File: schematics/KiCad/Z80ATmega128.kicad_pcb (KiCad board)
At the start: 2 copper layers, 97 parts, among them J1 AVR-ISP-6, J2 DC 5V, J3 DC 5V, J4 Z80[1..20], J5 Z80[21..40], J6 Micro_SD_Card_Det_Hirose_DM3AT, SW1 POWER, SW2 RESET, SW3 RESET, U1 74HC125, U10 AE-CH340E-TYPEC, U11 74HC08, U12 74HC32, U13 74HC74, U14 DS1232, U15 74HC132, U16 74HC4050, U17 LP2950-3.3, U2 74AC573, U3 74HCT574, U4 74HC04, U5 AE-CH340E-TYPEC, U6 74HC125, U7 74HC244, U8 74HCT245, U9 74HC32, Y1 16MHz, Y2 8MHz

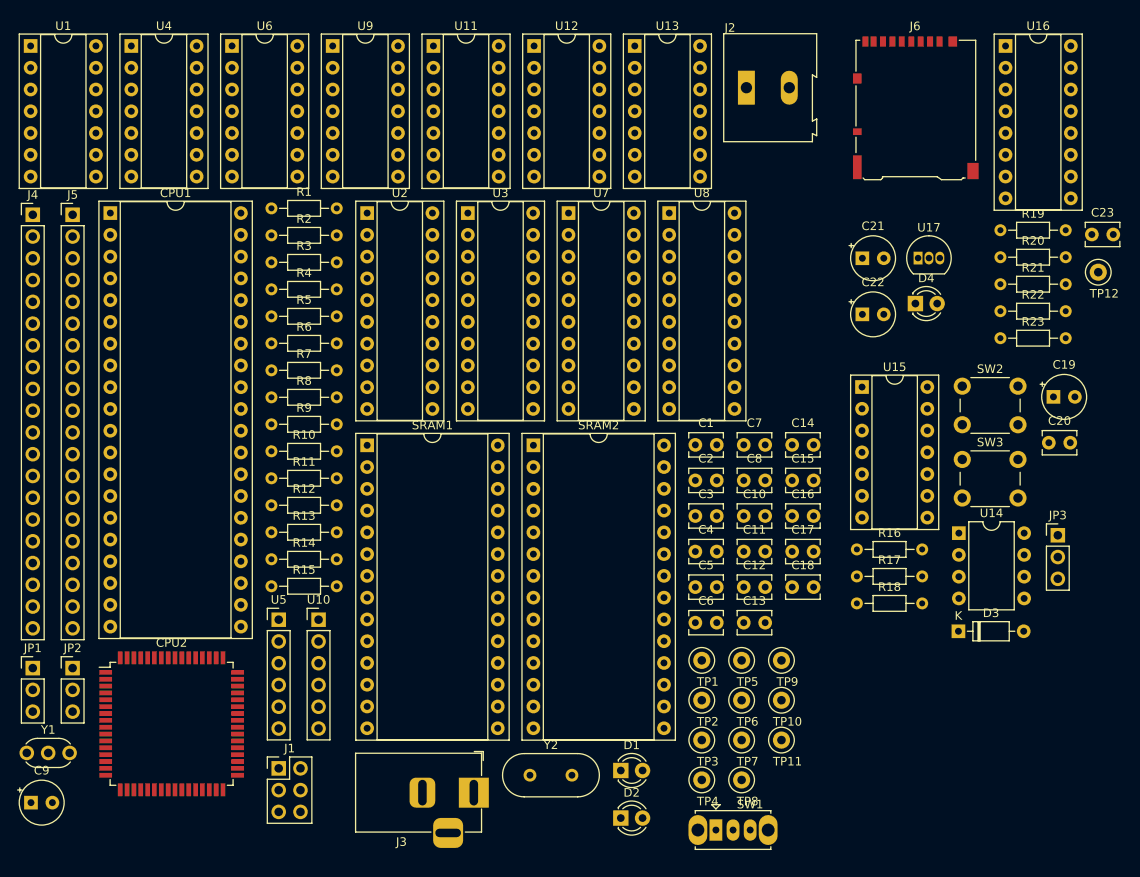
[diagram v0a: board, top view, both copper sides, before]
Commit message: Update schematics.
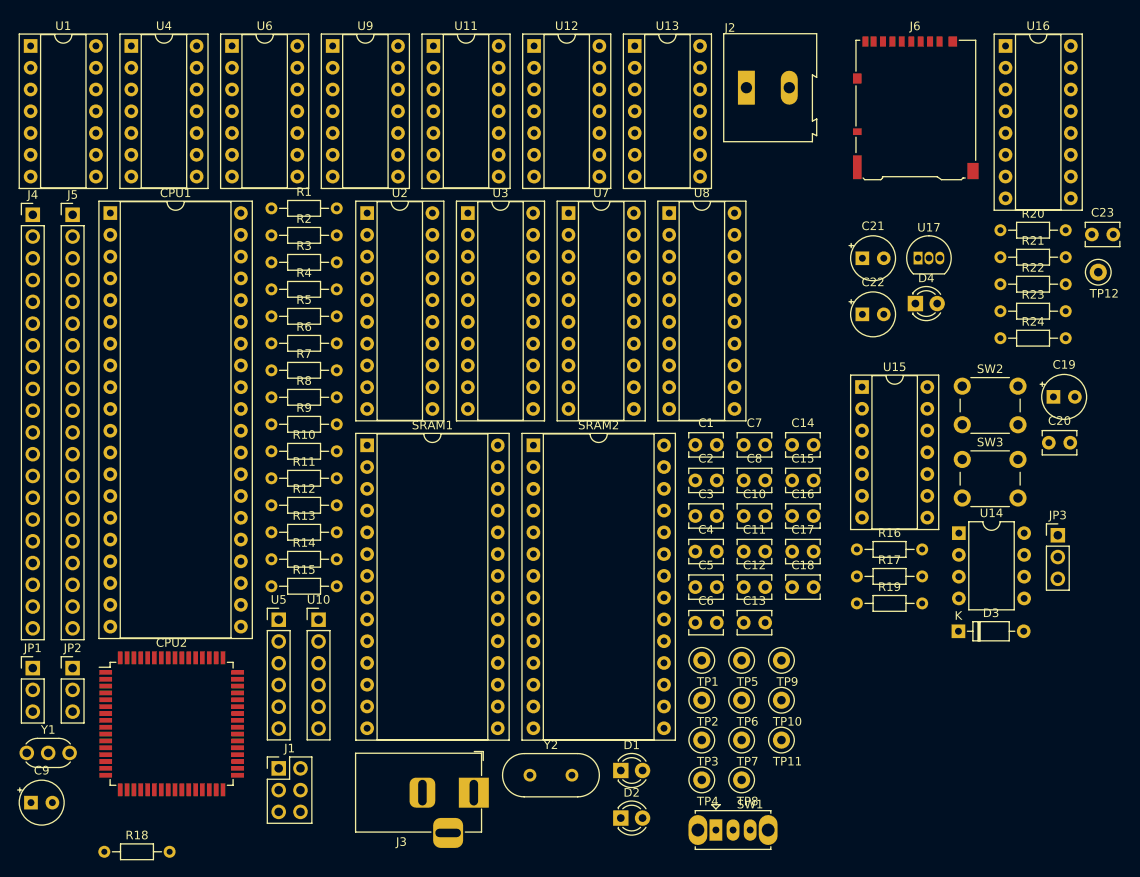
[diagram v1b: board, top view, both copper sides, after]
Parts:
- added R18: 10K, Resistor_THT:R_Axial_DIN0204_L3.6mm_D1.6mm_P7.62mm_Horizontal, F.Cu at (36.8, 121.9)
- renumbered R18 to R19, R19 to R20, R20 to R21, R21 to R22, R22 to R23, R23 to R24
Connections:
- U14 pad 2: GND -> VCC
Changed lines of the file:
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@@
   (net 101 "unconnected-(J6-DAT1-Pad8)")
   (net 102 "unconnected-(J6-SHIELD-Pad11)")
-  (net 103 "Net-(#FLG01-pwr)")
+  (net 103 "Net-(JP2-C)")
   (net 104 "Net-(JP3-A)")
   (net 105 "Net-(JP3-C)")
   (net 106 "Net-(JP3-B)")
   (net 107 "Net-(R14-Pad2)")
-  (net 108 "Net-(R18-Pad1)")
-  (net 109 "Net-(R23-Pad1)")
+  (net 108 "Net-(R19-Pad1)")
+  (net 109 "Net-(R24-Pad1)")
   (net 110 "Net-(SRAM1-~{OE})")
   (net 111 "Net-(SRAM1-~{WE})")
@@
     (property "ki_keywords" "R res resistor")
     (attr through_hole)
-    (fp_text reference "R22" (at 3.81 -1.92) (layer "F.SilkS")
+    (fp_text reference "R23" (at 3.81 -1.92) (layer "F.SilkS")
         (effects (font (size 1 1) (thickness 0.15)))
     )
@@
     (property "ki_keywords" "R res resistor")
     (attr through_hole)
-    (fp_text reference "R20" (at 3.81 -1.92) (layer "F.SilkS")
+    (fp_text reference "R21" (at 3.81 -1.92) (layer "F.SilkS")
         (effects (font (size 1 1) (thickness 0.15)))
     )
@@
       (net 114 "Net-(U14-{slash}PBRST)") (pinfunction "/PBRST") (pintype "input"))
     (pad "2" thru_hole oval (at 0 2.54) (size 1.6 1.6) (drill 0.8) (layers "*.Cu" "*.Mask")
-      (net 1 "GND") (pinfunction "TD") (pintype "input"))
+      (net 2 "VCC") (pinfunction "TD") (pintype "input"))
     (pad "3" thru_hole oval (at 0 5.08) (size 1.6 1.6) (drill 0.8) (layers "*.Cu" "*.Mask")
       (net 1 "GND") (pinfunction "TOL") (pintype "input"))
@@
     (property "ki_keywords" "R res resistor")
     (attr through_hole)
-    (fp_text reference "R19" (at 3.81 -1.92) (layer "F.SilkS")
+    (fp_text reference "R20" (at 3.81 -1.92) (layer "F.SilkS")
         (effects (font (size 1 1) (thickness 0.15)))
     )
@@
     (property "ki_keywords" "R res resistor")
     (attr through_hole)
-    (fp_text reference "R23" (at 3.81 -1.92) (layer "F.SilkS")
+    (fp_text reference "R24" (at 3.81 -1.92) (layer "F.SilkS")
         (effects (font (size 1 1) (thickness 0.15)))
     )
@@
       (stroke (width 0.1) (type solid)) (layer "F.Fab"))
     (pad "1" thru_hole circle (at 0 0) (size 1.4 1.4) (drill 0.7) (layers "*.Cu" "*.Mask")
-      (net 109 "Net-(R23-Pad1)") (pintype "passive"))
+      (net 109 "Net-(R24-Pad1)") (pintype "passive"))
     (pad "2" thru_hole oval (at 7.62 0) (size 1.4 1.4) (drill 0.7) (layers "*.Cu" "*.Mask")
       (net 93 "Net-(D4-A)") (pintype "passive"))
@@
       (net 55 "SCK") (pintype "input"))
     (pad "10" thru_hole oval (at 7.62 15.24) (size 1.6 1.6) (drill 0.8) (layers "*.Cu" "*.Mask")
-      (net 109 "Net-(R23-Pad1)") (pintype "output"))
+      (net 109 "Net-(R24-Pad1)") (pintype "output"))
     (pad "11" thru_hole oval (at 7.62 12.7) (size 1.6 1.6) (drill 0.8) (layers "*.Cu" "*.Mask")
       (net 1 "GND") (pintype "input"))
@@
     )
   )
+  (footprint "Resistor_THT:R_Axial_DIN0204_L3.6mm_D1.6mm_P7.62mm_Horizontal" (layer "F.Cu")
+    (at 36.83 121.92)
+    (descr "Resistor, Axial_DIN0204 series, Axial, Horizontal, pin pitch=7.62mm, 0.167W, length*diameter=3.6*1.6mm^2, http://cdn-reichelt.de/documents/datenblatt/B400/1_4W%23YAG.pdf")
+    (tags "Resistor Axial_DIN0204 series Axial Horizontal pin pitch 7.62mm 0.167W length 3.6mm diameter 1.6mm")
+    (property "Sheetfile" "Reset.kicad_sch")
+    (property "Sheetname" "Reset")
+    (property "ki_description" "Resistor")
+    (property "ki_keywords" "R res resistor")
+    (attr through_hole)
+    (fp_text reference "R18" (at 3.81 -1.92) (layer "F.SilkS")
+        (effects (font (size 1 1) (thickness 0.15)))
+    )
+    (fp_text value "10K" (at 3.81 1.92) (layer "F.Fab")
+        (effects (font (size 1 1) (thickness 0.15)))
+    )
+    (fp_text user "${REFERENCE}" (at 3.81 0) (layer "F.Fab")
+        (effects (font (size 0.72 0.72) (thickness 0.108)))
+    )
+    (fp_line (start 0.94 0) (end 1.89 0)
+      (stroke (width 0.12) (type solid)) (layer "F.SilkS"))
+    (fp_line (start 1.89 -0.92) (end 1.89 0.92)
+      (stroke (width 0.12) (type solid)) (layer "F.SilkS"))
+    (fp_line (start 1.89 0.92) (end 5.73 0.92)
+      (stroke (width 0.12) (type solid)) (layer "F.SilkS"))
+    (fp_line (start 5.73 -0.92) (end 1.89 -0.92)
+      (stroke (width 0.12) (type solid)) (layer "F.SilkS"))
+    (fp_line (start 5.73 0.92) (end 5.73 -0.92)
+      (stroke (width 0.12) (type solid)) (layer "F.SilkS"))
+    (fp_line (start 6.68 0) (end 5.73 0)
+      (stroke (width 0.12) (type solid)) (layer "F.SilkS"))
+    (fp_line (start -0.95 -1.05) (end -0.95 1.05)
+      (stroke (width 0.05) (type solid)) (layer "F.CrtYd"))
+    (fp_line (start -0.95 1.05) (end 8.57 1.05)
+      (stroke (width 0.05) (type solid)) (layer "F.CrtYd"))
+    (fp_line (start 8.57 -1.05) (end -0.95 -1.05)
+      (stroke (width 0.05) (type solid)) (layer "F.CrtYd"))
+    (fp_line (start 8.57 1.05) (end 8.57 -1.05)
+      (stroke (width 0.05) (type solid)) (layer "F.CrtYd"))
+    (fp_line (start 0 0) (end 2.01 0)
+      (stroke (width 0.1) (type solid)) (layer "F.Fab"))
+    (fp_line (start 2.01 -0.8) (end 2.01 0.8)
+      (stroke (width 0.1) (type solid)) (layer "F.Fab"))
+    (fp_line (start 2.01 0.8) (end 5.61 0.8)
+      (stroke (width 0.1) (type solid)) (layer "F.Fab"))
+    (fp_line (start 5.61 -0.8) (end 2.01 -0.8)
+      (stroke (width 0.1) (type solid)) (layer "F.Fab"))
+    (fp_line (start 5.61 0.8) (end 5.61 -0.8)
+      (stroke (width 0.1) (type solid)) (layer "F.Fab"))
+    (fp_line (start 7.62 0) (end 5.61 0)
+      (stroke (width 0.1) (type solid)) (layer "F.Fab"))
+    (pad "1" thru_hole circle (at 0 0) (size 1.4 1.4) (drill 0.7) (layers "*.Cu" "*.Mask")
+      (net 59 "/Reset/{slash}Z80_SWRST") (pintype "passive"))
+    (pad "2" thru_hole oval (at 7.62 0) (size 1.4 1.4) (drill 0.7) (layers "*.Cu" "*.Mask")
+      (net 2 "VCC") (pintype "passive"))
+    (model "${KICAD6_3DMODEL_DIR}/Resistor_THT.3dshapes/R_Axial_DIN0204_L3.6mm_D1.6mm_P7.62mm_Horizontal.wrl"
+      (offset (xyz 0 0 0))
+      (scale (xyz 1 1 1))
+      (rotate (xyz 0 0 0))
+    )
+  )
   (footprint "Connector_PinHeader_2.54mm:PinHeader_1x06_P2.54mm_Vertical" (layer "F.Cu")
     (at 61.83 94.835)
@@
       (net 67 "RXD1") (pinfunction "TXD") (pintype "output"))
     (pad "4" thru_hole oval (at 0 7.62) (size 1.7 1.7) (drill 1) (layers "*.Cu" "*.Mask")
-      (net 103 "Net-(#FLG01-pwr)") (pinfunction "VCC") (pintype "power_in"))
+      (net 103 "Net-(JP2-C)") (pinfunction "VCC") (pintype "power_in"))
     (pad "5" thru_hole oval (at 0 10.16) (size 1.7 1.7) (drill 1) (layers "*.Cu" "*.Mask")
       (net 131 "unconnected-(U10-CTS-Pad5)") (pinfunction "CTS") (pintype "input+no_connect"))
@@
       (net 113 "unconnected-(SW1-A-Pad1)") (pinfunction "A") (pintype "passive+no_connect"))
     (pad "2" thru_hole oval (at 2 0) (size 1.5 2.5) (drill 0.8) (layers "*.Cu" "*.Mask")
-      (net 103 "Net-(#FLG01-pwr)") (pinfunction "B") (pintype "passive"))
+      (net 103 "Net-(JP2-C)") (pinfunction "B") (pintype "passive"))
     (pad "3" thru_hole oval (at 4 0) (size 1.5 2.5) (drill 0.8) (layers "*.Cu" "*.Mask")
       (net 2 "VCC") (pinfunction "C") (pintype "passive"))
@@
       (net 1 "GND") (pinfunction "1") (pintype "passive"))
     (pad "2" thru_hole circle (at 0 4.5 90) (size 2 2) (drill 1.1) (layers "*.Cu" "*.Mask")
-      (net 108 "Net-(R18-Pad1)") (pinfunction "2") (pintype "passive"))
+      (net 108 "Net-(R19-Pad1)") (pinfunction "2") (pintype "passive"))
     (pad "2" thru_hole circle (at 6.5 4.5 90) (size 2 2) (drill 1.1) (layers "*.Cu" "*.Mask")
-      (net 108 "Net-(R18-Pad1)") (pinfunction "2") (pintype "passive"))
+      (net 108 "Net-(R19-Pad1)") (pinfunction "2") (pintype "passive"))
     (model "${KICAD6_3DMODEL_DIR}/Button_Switch_THT.3dshapes/SW_PUSH_6mm_H7.3mm.wrl"
       (offset (xyz 0 0 0))
@@
       (net 97 "Net-(J3-In)") (pinfunction "A") (pintype "passive"))
     (pad "2" thru_hole oval (at 0 2.54) (size 1.7 1.7) (drill 1) (layers "*.Cu" "*.Mask")
-      (net 103 "Net-(#FLG01-pwr)") (pinfunction "C") (pintype "passive"))
+      (net 103 "Net-(JP2-C)") (pinfunction "C") (pintype "passive"))
     (pad "3" thru_hole oval (at 0 5.08) (size 1.7 1.7) (drill 1) (layers "*.Cu" "*.Mask")
       (net 96 "Net-(J2-Pin_2)") (pinfunction "B") (pintype "passive"))
@@
     (property "ki_keywords" "R res resistor")
     (attr through_hole)
-    (fp_text reference "R18" (at 3.81 -1.92) (layer "F.SilkS")
+    (fp_text reference "R19" (at 3.81 -1.92) (layer "F.SilkS")
         (effects (font (size 1 1) (thickness 0.15)))
     )
@@
       (stroke (width 0.1) (type solid)) (layer "F.Fab"))
     (pad "1" thru_hole circle (at 0 0) (size 1.4 1.4) (drill 0.7) (layers "*.Cu" "*.Mask")
-      (net 108 "Net-(R18-Pad1)") (pintype "passive"))
+      (net 108 "Net-(R19-Pad1)") (pintype "passive"))
     (pad "2" thru_hole oval (at 7.62 0) (size 1.4 1.4) (drill 0.7) (layers "*.Cu" "*.Mask")
       (net 5 "Net-(D3-A)") (pintype "passive"))
@@
     (property "ki_keywords" "R res resistor")
     (attr through_hole)
-    (fp_text reference "R21" (at 3.81 -1.92) (layer "F.SilkS")
+    (fp_text reference "R22" (at 3.81 -1.92) (layer "F.SilkS")
         (effects (font (size 1 1) (thickness 0.15)))
     )
@@
       (net 124 "Net-(U5-TXD)") (pinfunction "TXD") (pintype "output"))
     (pad "4" thru_hole oval (at 0 7.62) (size 1.7 1.7) (drill 1) (layers "*.Cu" "*.Mask")
-      (net 103 "Net-(#FLG01-pwr)") (pinfunction "VCC") (pintype "power_in"))
+      (net 103 "Net-(JP2-C)") (pinfunction "VCC") (pintype "power_in"))
     (pad "5" thru_hole oval (at 0 10.16) (size 1.7 1.7) (drill 1) (layers "*.Cu" "*.Mask")
       (net 125 "unconnected-(U5-CTS-Pad5)") (pinfunction "CTS") (pintype "input+no_connect"))
